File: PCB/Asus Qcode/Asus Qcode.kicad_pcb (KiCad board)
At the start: 2 copper layers, 67.3 x 49.5 mm, 14 parts, among them J1 COM_DEBUG, J2 Conn_01x03_Pin, J3 Conn_01x02_Pin, SW1 Recall Codes

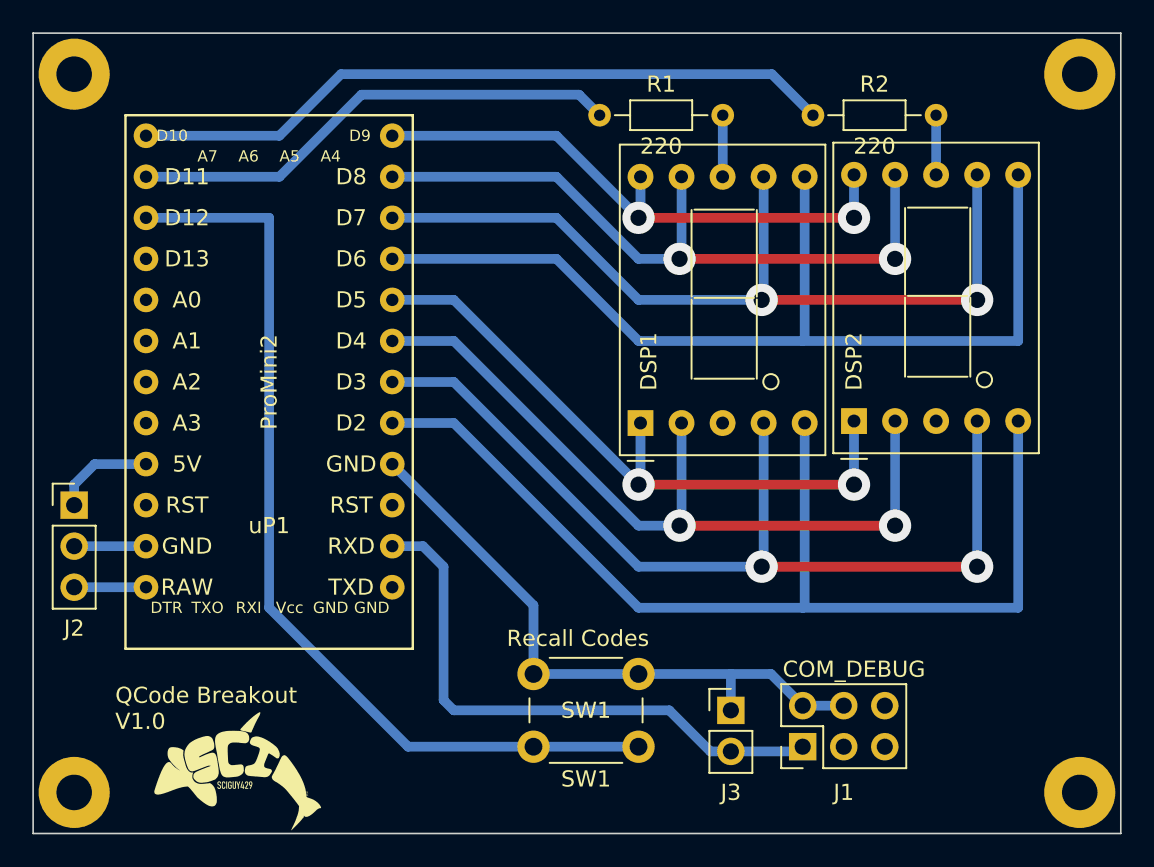
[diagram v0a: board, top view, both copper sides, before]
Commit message: More PCB Tweaks
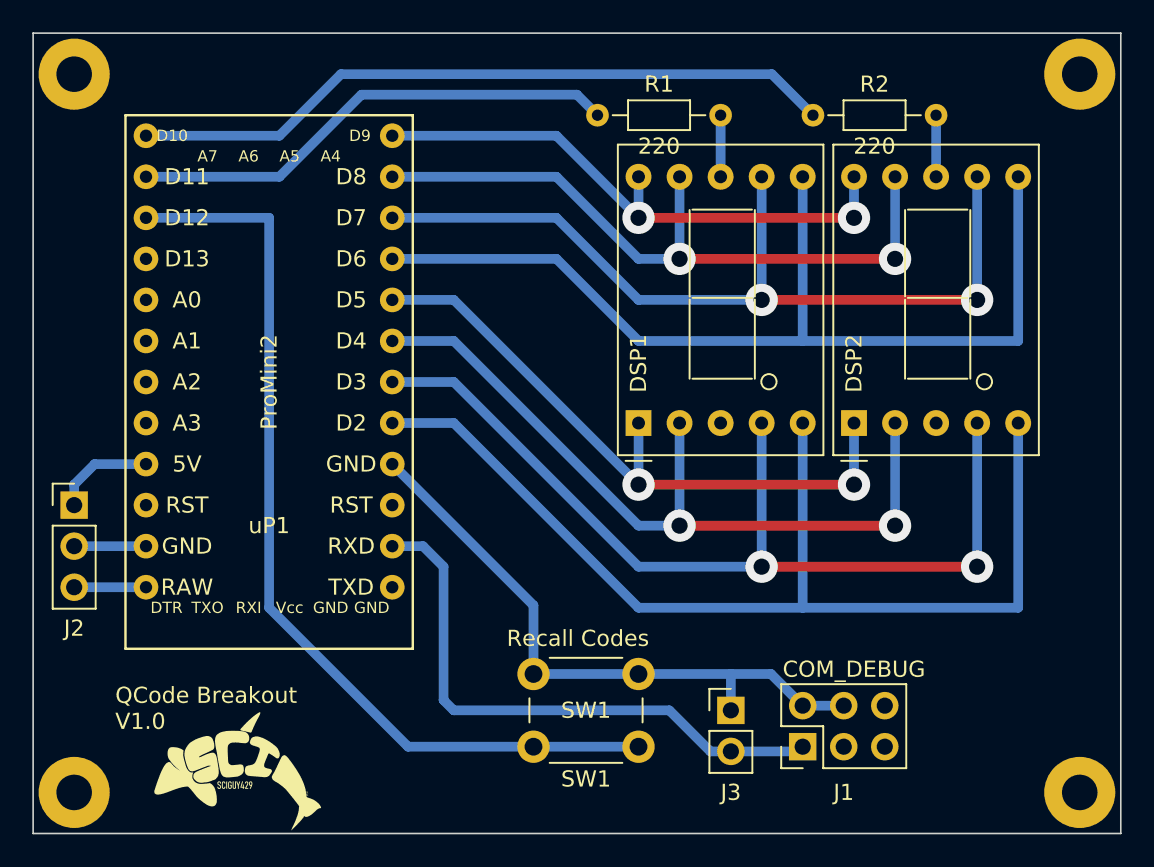
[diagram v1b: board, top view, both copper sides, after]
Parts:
- moved R1 0.13 mm to (47.6, 17.8)
- moved DSP1 0.12 mm to (50.2, 36.8)
- moved DSP2 0.12 mm to (63.5, 36.8)
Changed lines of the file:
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@@
   )
   (footprint "Resistor_THT:R_Axial_DIN0204_L3.6mm_D1.6mm_P7.62mm_Horizontal" (layer "F.Cu")
-    (at 47.756627 17.78)
+    (at 47.625 17.78)
     (descr "Resistor, Axial_DIN0204 series, Axial, Horizontal, pin pitch=7.62mm, 0.167W, length*diameter=3.6*1.6mm^2, http://cdn-reichelt.de/documents/datenblatt/B400/1_4W%23YAG.pdf")
     (tags "Resistor Axial_DIN0204 series Axial Horizontal pin pitch 7.62mm 0.167W length 3.6mm diameter 1.6mm")
@@
   )
   (footprint "Display_7Segment:D1X8K" (layer "F.Cu")
-    (at 63.5 36.7075 90)
+    (at 63.5 36.83 90)
     (descr "https://ia800903.us.archive.org/24/items/CTKD1x8K/Cromatek%20D168K.pdf")
     (tags "Single digit 7 segment ultra bright red")
@@
   )
   (footprint "Display_7Segment:D1X8K" (layer "F.Cu")
-    (at 50.2875 36.83 90)
+    (at 50.165 36.83 90)
     (descr "https://ia800903.us.archive.org/24/items/CTKD1x8K/Cromatek%20D168K.pdf")
     (tags "Single digit 7 segment ultra bright red")
@@
     (property "ki_keywords" "display LED 7-segment")
     (attr through_hole)
-    (fp_text reference "DSP1" (at 3.81 0.5125 90) (layer "F.SilkS")
+    (fp_text reference "DSP1" (at 3.6875 0 90) (layer "F.SilkS")
         (effects (font (size 1 1) (thickness 0.15)))
     )
@@
   (via (at 63.5 40.64) (size 2) (drill 1) (layers "F.Cu" "B.Cu") (net 1))
   (segment (start 34.925 29.21) (end 38.735 29.21) (width 0.6) (layer "B.Cu") (net 1))
+  (segment (start 50.165 36.83) (end 50.165 40.64) (width 0.6) (layer "B.Cu") (net 1))
   (segment (start 63.5 40.64) (end 63.5 36.7075) (width 0.6) (layer "B.Cu") (net 1))
   (segment (start 50.165 40.64) (end 50.2875 40.5175) (width 0.6) (layer "B.Cu") (net 1))
-  (segment (start 50.2875 40.5175) (end 50.2875 36.83) (width 0.6) (layer "B.Cu") (net 1))
   (segment (start 38.735 29.21) (end 50.165 40.64) (width 0.6) (layer "B.Cu") (net 1))
   (segment (start 52.705 43.18) (end 66.04 43.18) (width 0.6) (layer "F.Cu") (net 2))
@@
   (segment (start 34.925 31.75) (end 38.735 31.75) (width 0.6) (layer "B.Cu") (net 2))
   (segment (start 50.165 43.18) (end 52.705 43.18) (width 0.6) (layer "B.Cu") (net 2))
+  (segment (start 52.705 36.83) (end 52.705 43.18) (width 0.6) (layer "B.Cu") (net 2))
   (segment (start 66.04 43.18) (end 66.04 36.7075) (width 0.6) (layer "B.Cu") (net 2))
-  (segment (start 52.8275 43.0575) (end 52.8275 36.83) (width 0.6) (layer "B.Cu") (net 2))
   (segment (start 38.735 31.75) (end 50.165 43.18) (width 0.6) (layer "B.Cu") (net 2))
-  (segment (start 55.376627 17.78) (end 55.376627 21.580873) (width 0.6) (layer "B.Cu") (net 3))
+  (segment (start 55.245 17.78) (end 55.245 21.59) (width 0.6) (layer "B.Cu") (net 3))
   (segment (start 55.376627 21.580873) (end 55.3675 21.59) (width 0.6) (layer "B.Cu") (net 3))
   (segment (start 57.785 45.72) (end 71.12 45.72) (width 0.6) (layer "F.Cu") (net 4))
@@
   (via (at 57.785 45.72) (size 2) (drill 1) (layers "F.Cu" "B.Cu") (net 4))
   (segment (start 34.925 34.29) (end 38.735 34.29) (width 0.6) (layer "B.Cu") (net 4))
+  (segment (start 57.785 36.83) (end 57.785 45.72) (width 0.6) (layer "B.Cu") (net 4))
   (segment (start 71.12 45.72) (end 71.12 36.7075) (width 0.6) (layer "B.Cu") (net 4))
   (segment (start 57.785 45.72) (end 57.9075 45.5975) (width 0.6) (layer "B.Cu") (net 4))
   (segment (start 38.735 34.29) (end 50.165 45.72) (width 0.6) (layer "B.Cu") (net 4))
   (segment (start 50.165 45.72) (end 57.785 45.72) (width 0.6) (layer "B.Cu") (net 4))
-  (segment (start 57.9075 45.5975) (end 57.9075 36.83) (width 0.6) (layer "B.Cu") (net 4))
   (segment (start 38.735 36.83) (end 50.165 48.26) (width 0.6) (layer "B.Cu") (net 5))
-  (segment (start 60.4475 48.1375) (end 60.4475 36.83) (width 0.6) (layer "B.Cu") (net 5))
+  (segment (start 60.325 36.83) (end 60.325 48.26) (width 0.6) (layer "B.Cu") (net 5))
   (segment (start 73.66 48.26) (end 73.66 36.7075) (width 0.6) (layer "B.Cu") (net 5))
   (segment (start 50.165 48.26) (end 60.325 48.26) (width 0.6) (layer "B.Cu") (net 5))
-  (segment (start 60.325 48.26) (end 60.4475 48.1375) (width 0.6) (layer "B.Cu") (net 5))
   (segment (start 34.925 36.83) (end 38.735 36.83) (width 0.6) (layer "B.Cu") (net 5))
   (segment (start 60.325 48.26) (end 73.66 48.26) (width 0.6) (layer "B.Cu") (net 5))
-  (segment (start 60.325 31.75) (end 60.4475 31.6275) (width 0.6) (layer "B.Cu") (net 6))
   (segment (start 34.925 26.67) (end 45.085 26.67) (width 0.6) (layer "B.Cu") (net 6))
-  (segment (start 60.4475 31.6275) (end 60.4475 21.59) (width 0.6) (layer "B.Cu") (net 6))
   (segment (start 73.66 31.75) (end 73.66 21.4675) (width 0.6) (layer "B.Cu") (net 6))
   (segment (start 50.165 31.75) (end 60.325 31.75) (width 0.6) (layer "B.Cu") (net 6))
   (segment (start 45.085 26.67) (end 50.165 31.75) (width 0.6) (layer "B.Cu") (net 6))
   (segment (start 60.325 31.75) (end 73.66 31.75) (width 0.6) (layer "B.Cu") (net 6))
+  (segment (start 60.325 21.59) (end 60.325 31.75) (width 0.6) (layer "B.Cu") (net 6))
   (segment (start 57.785 29.21) (end 71.12 29.21) (width 0.6) (layer "F.Cu") (net 7))
   (via (at 57.785 29.21) (size 2) (drill 1) (layers "F.Cu" "B.Cu") (net 7))
@@
   (segment (start 34.925 24.13) (end 45.085 24.13) (width 0.6) (layer "B.Cu") (net 7))
   (segment (start 50.165 29.21) (end 57.785 29.21) (width 0.6) (layer "B.Cu") (net 7))
-  (segment (start 57.9075 29.0875) (end 57.9075 21.59) (width 0.6) (layer "B.Cu") (net 7))
+  (segment (start 57.785 21.59) (end 57.785 29.21) (width 0.6) (layer "B.Cu") (net 7))
   (segment (start 71.12 29.21) (end 71.12 21.4675) (width 0.6) (layer "B.Cu") (net 7))
   (segment (start 52.705 26.67) (end 66.04 26.67) (width 0.6) (layer "F.Cu") (net 8))
   (via (at 52.705 26.67) (size 2) (drill 1) (layers "F.Cu" "B.Cu") (net 8))
   (via (at 66.04 26.67) (size 2) (drill 1) (layers "F.Cu" "B.Cu") (net 8))
-  (segment (start 52.8275 26.5475) (end 52.8275 21.59) (width 0.6) (layer "B.Cu") (net 8))
   (segment (start 52.705 26.67) (end 52.8275 26.5475) (width 0.6) (layer "B.Cu") (net 8))
   (segment (start 50.165 26.67) (end 52.705 26.67) (width 0.6) (layer "B.Cu") (net 8))
   (segment (start 66.04 26.67) (end 66.04 21.4675) (width 0.6) (layer "B.Cu") (net 8))
+  (segment (start 52.705 21.59) (end 52.705 26.67) (width 0.6) (layer "B.Cu") (net 8))
   (segment (start 45.085 21.59) (end 50.165 26.67) (width 0.6) (layer "B.Cu") (net 8))
   (segment (start 34.925 21.59) (end 45.085 21.59) (width 0.6) (layer "B.Cu") (net 8))
@@
   (via (at 50.165 24.13) (size 2) (drill 1) (layers "F.Cu" "B.Cu") (net 9))
   (via (at 63.5 24.13) (size 2) (drill 1) (layers "F.Cu" "B.Cu") (net 9))
+  (segment (start 50.165 21.59) (end 50.165 24.13) (width 0.6) (layer "B.Cu") (net 9))
   (segment (start 63.5 24.13) (end 63.5 21.4675) (width 0.6) (layer "B.Cu") (net 9))
   (segment (start 50.165 24.13) (end 50.2875 24.0075) (width 0.6) (layer "B.Cu") (net 9))
   (segment (start 45.085 19.05) (end 50.165 24.13) (width 0.6) (layer "B.Cu") (net 9))
   (segment (start 34.925 19.05) (end 45.085 19.05) (width 0.6) (layer "B.Cu") (net 9))
-  (segment (start 50.2875 24.0075) (end 50.2875 21.59) (width 0.6) (layer "B.Cu") (net 9))
   (segment (start 68.58 17.78) (end 68.58 21.4675) (width 0.6) (layer "B.Cu") (net 10))
   (segment (start 35.905 56.86) (end 27.305 48.26) (width 0.6) (layer "B.Cu") (net 13))
@@
   (segment (start 15.24 44.45) (end 19.685 44.45) (width 0.6) (layer "B.Cu") (net 27))
   (segment (start 15.24 46.99) (end 19.685 46.99) (width 0.6) (layer "B.Cu") (net 28))
-  (segment (start 33.02 16.51) (end 46.486627 16.51) (width 0.6) (layer "B.Cu") (net 29))
   (segment (start 27.94 21.59) (end 33.02 16.51) (width 0.6) (layer "B.Cu") (net 29))
-  (segment (start 46.486627 16.51) (end 47.756627 17.78) (width 0.6) (layer "B.Cu") (net 29))
+  (segment (start 46.355 16.51) (end 47.625 17.78) (width 0.6) (layer "B.Cu") (net 29))
   (segment (start 19.685 21.59) (end 27.94 21.59) (width 0.6) (layer "B.Cu") (net 29))
+  (segment (start 33.02 16.51) (end 46.355 16.51) (width 0.6) (layer "B.Cu") (net 29))
   (segment (start 58.42 15.24) (end 60.96 17.78) (width 0.6) (layer "B.Cu") (net 30))
   (segment (start 19.685 19.05) (end 27.94 19.05) (width 0.6) (layer "B.Cu") (net 30))
